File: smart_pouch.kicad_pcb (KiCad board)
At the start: 2 copper layers, 92 parts, among them CN1 B3B-PH-K-S, J1 XH-2P-SMD, J2 2.54-3P-LT, J3 SIM_Card, Q2 PMV20XNER, Q3 2N7002, SW1 SW_Push, U1 nRF52840, U10 BWU.FL-IPEX1, U11 HX PZ1.27-2x5P TP, U12 MT3608, U13 MT3608, U14 HX PZ1.27-2x5P TP, U2 NRF9151-LACA-R7, U3 NPM1300, U4 BMA400, U5 DRV8871DDA, U6 BWU.FL-IPEX1, U7 AN6520-245, U8 SEN0348_CONN, U9 XH-4A, Y1 32MHz

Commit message: Initial PCB commit
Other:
- copper layers 2 -> 4
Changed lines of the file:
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@@
 	(layers
 		(0 "F.Cu" signal)
+		(4 "In1.Cu" signal)
+		(6 "In2.Cu" signal)
 		(2 "B.Cu" signal)
 		(9 "F.Adhes" user "F.Adhesive")
@@
 	)
 	(setup
+		(stackup
+			(layer "F.SilkS"
+				(type "Top Silk Screen")
+			)
+			(layer "F.Paste"
+				(type "Top Solder Paste")
+			)
+			(layer "F.Mask"
+				(type "Top Solder Mask")
+				(thickness 0.01)
+			)
+			(layer "F.Cu"
+				(type "copper")
+				(thickness 0.035)
+			)
+			(layer "dielectric 1"
+				(type "prepreg")
+				(color "FR4 natural")
+				(thickness 0.0994)
+				(material "3313")
+				(epsilon_r 4.1)
+				(loss_tangent 0.02)
+			)
+			(layer "In1.Cu"
+				(type "copper")
+				(thickness 0.0152)
+			)
+			(layer "dielectric 2"
+				(type "core")
+				(color "FR4 natural")
+				(thickness 1.265)
+				(material "FR4")
+				(epsilon_r 4.6)
+				(loss_tangent 0.02)
+			)
+			(layer "In2.Cu"
+				(type "copper")
+				(thickness 0.0152)
+			)
+			(layer "dielectric 3"
+				(type "prepreg")
+				(color "FR4 natural")
+				(thickness 0.0994)
+				(material "3313")
+				(epsilon_r 4.1)
+				(loss_tangent 0.02)
+			)
+			(layer "B.Cu"
+				(type "copper")
+				(thickness 0.035)
+			)
+			(layer "B.Mask"
+				(type "Bottom Solder Mask")
+				(thickness 0.01)
+			)
+			(layer "B.Paste"
+				(type "Bottom Solder Paste")
+			)
+			(layer "B.SilkS"
+				(type "Bottom Silk Screen")
+			)
+			(copper_finish "ENIG")
+			(dielectric_constraints yes)
+		)
 		(pad_to_mask_clearance 0)
 		(allow_soldermask_bridges_in_footprints no)

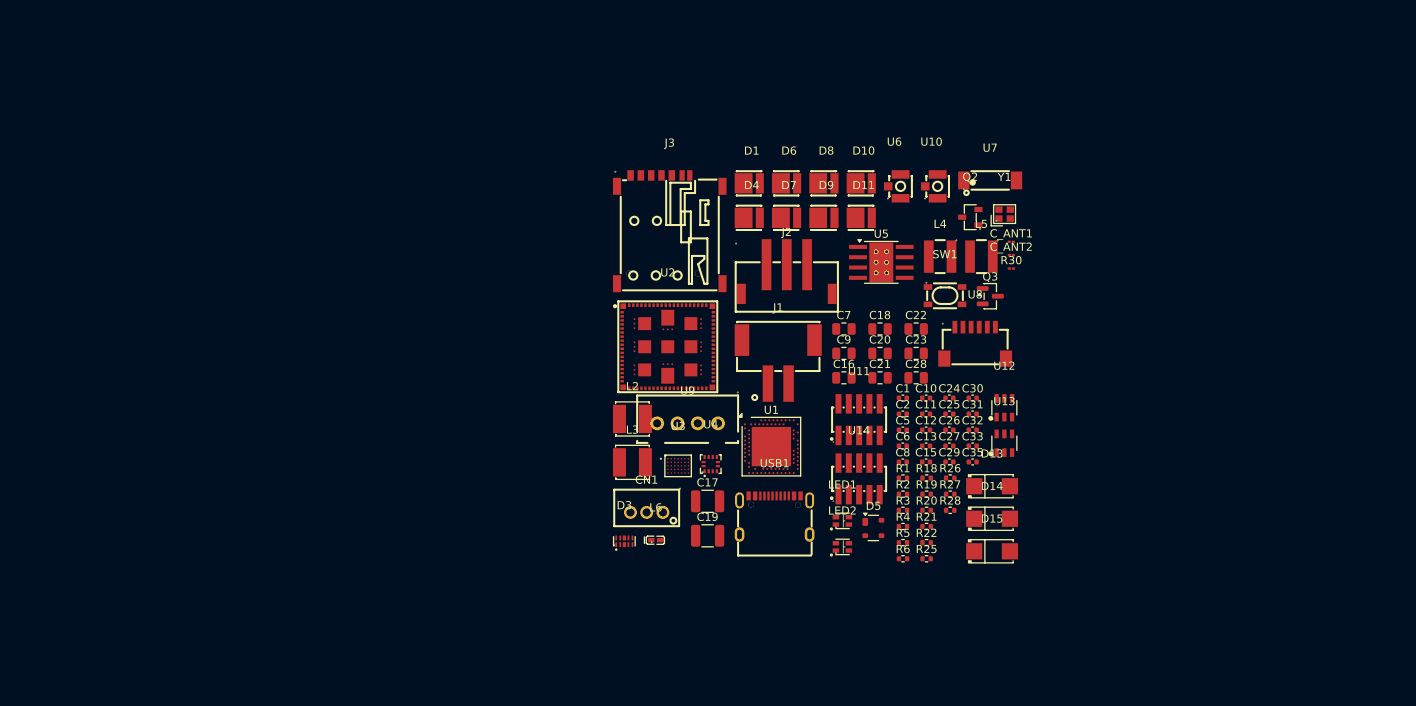
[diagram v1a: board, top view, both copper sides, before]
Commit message: pcb basic layout
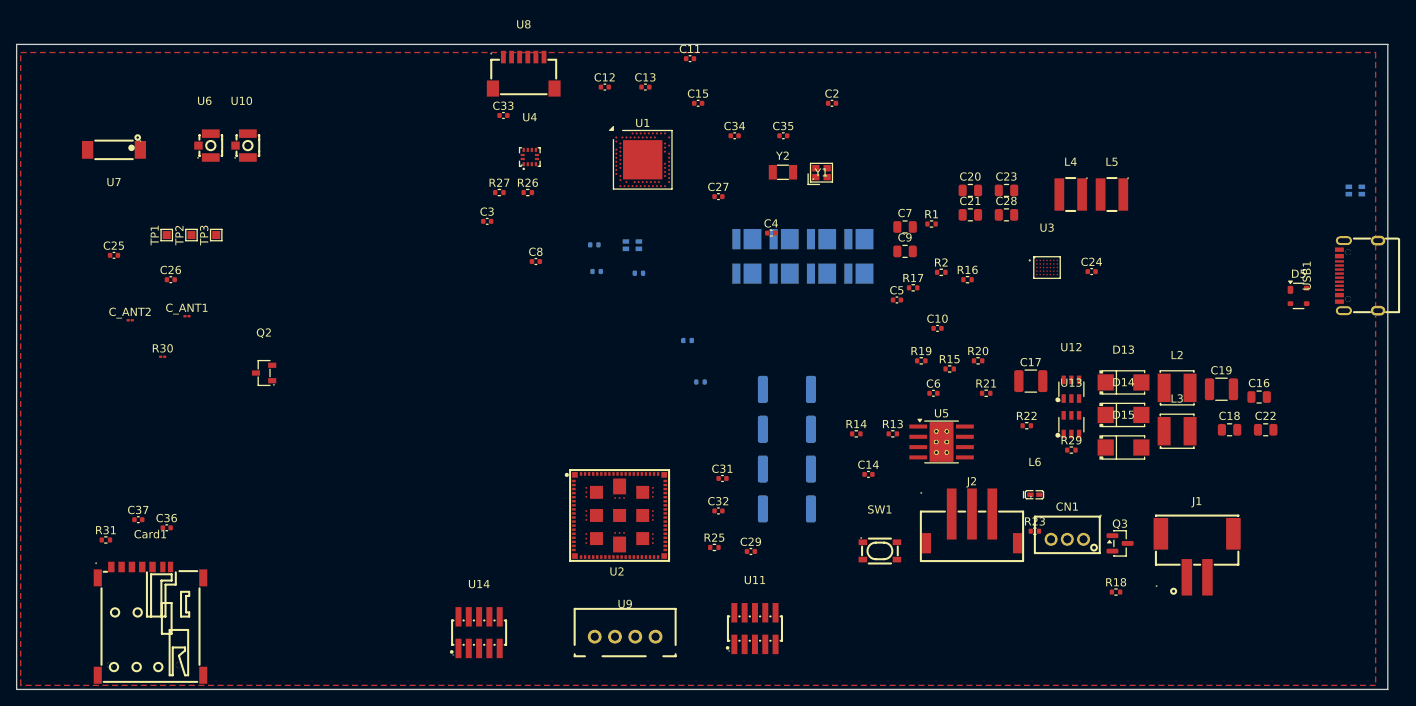
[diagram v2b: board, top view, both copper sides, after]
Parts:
- removed C1, C30: 100nF, Capacitor_SMD:C_0402_1005Metric
- removed D3: SP3012-04UTG, easyeda2kicad:UDFN-10_L2.5-W1.0-P0.50-BL
- removed J3: SIM_Card, easyeda2kicad:SIM-SMD_SMN-303
- removed R3, R4: 10k, Resistor_SMD:R_0402_1005Metric
- added C14: 100nF, Capacitor_SMD:C_0402_1005Metric, F.Cu at (154.0, 102.0)
- added C3: 100nF, Capacitor_SMD:C_0402_1005Metric, F.Cu at (107.0, 70.8)
- added C34: 12pF, Capacitor_SMD:C_0402_1005Metric, F.Cu at (137.5, 60.3)
- added C36: 100nF, Capacitor_SMD:C_0402_1005Metric, F.Cu at (67.5, 108.6)
- added C37: 100nF, Capacitor_SMD:C_0402_1005Metric, F.Cu at (64.0, 107.6)
- added C4: 12pF, Capacitor_SMD:C_0402_1005Metric, F.Cu at (142.0, 72.3)
- added Card1: SMN-303, easyeda2kicad:SIM-SMD_SMN-303, F.Cu at (65.5, 120.1)
- added R10: 39R, Resistor_SMD:R_2512_6332Metric, B.Cu at (143.9, 106.2)
- added R11: 150R, Resistor_SMD:R_0402_1005Metric, B.Cu at (133.3, 90.6)
- added R12: 10k, Resistor_SMD:R_0402_1005Metric, B.Cu at (131.7, 85.5)
- added R13: 560k, Resistor_SMD:R_0402_1005Metric, F.Cu at (157.0, 97.0)
- added R14: 2.2M, Resistor_SMD:R_0402_1005Metric, F.Cu at (152.5, 97.0)
- added R15: 100k, Resistor_SMD:R_0402_1005Metric, F.Cu at (164.0, 89.0)
- added R16: 10k, Resistor_SMD:R_0402_1005Metric, F.Cu at (166.2, 78.0)
- added R17: 10k, Resistor_SMD:R_0402_1005Metric, F.Cu at (159.5, 79.0)
- added R23: 18k, Resistor_SMD:R_0402_1005Metric, F.Cu at (174.5, 109.0)
- added R29: 100k, Resistor_SMD:R_0402_1005Metric, F.Cu at (179.0, 99.0)
- added R31: 10k, Resistor_SMD:R_0402_1005Metric, F.Cu at (60.0, 110.1)
- added R7: 39R, Resistor_SMD:R_2512_6332Metric, B.Cu at (143.9, 91.5)
- added R8: 39R, Resistor_SMD:R_2512_6332Metric, B.Cu at (143.9, 96.4)
- added R9: 39R, Resistor_SMD:R_2512_6332Metric, B.Cu at (143.9, 101.3)
- added TP1: TestPoint, TestPoint:TestPoint_Pad_1.0x1.0mm, F.Cu at (67.5, 72.5)
- added TP2: TestPoint, TestPoint:TestPoint_Pad_1.0x1.0mm, F.Cu at (70.5, 72.5)
- added TP3: TestPoint, TestPoint:TestPoint_Pad_1.0x1.0mm, F.Cu at (73.6, 72.5)
- added Y2: 32.768kHz, Crystal:Crystal_SMD_3215-2Pin_3.2x1.5mm, F.Cu at (143.4, 64.8)
- CN1: value B3B-PH-K-S -> JST 1x3 Battery P=1.27mm
- D1, D10, D11, D4, D6, D7, D8, D9, R28, R5, R6: moved to B.Cu
- D5: value PRTR5V0U2X -> PRTR5V0U2X ESD
- J1: value XH-2P-SMD -> Solenoid XH-2P-SMD
- J2: value 2.54-3P-LT -> 2.54-3P-LT Piezo
- LED1: value 19-237/R6GHBHC-A01/2T -> Power RGB; moved to B.Cu
- LED2: value 19-237/R6GHBHC-A01/2T -> USER LED; moved to B.Cu
- U11: value HX PZ1.27-2x5P TP -> 9151 SWD P=1.27mm 2x5P
- U14: value HX PZ1.27-2x5P TP -> 52840 SWD P=1.27mm 2x5P
- U8: value SEN0348_CONN -> JST P=1mm 01x06
- U9: value XH-4A -> XH-4A UART 9151
- USB1: value TYPE-C 16PIN 2MD -> TYPE-C 16P
- moved C_ANT2 108.9 mm to (63.0, 83.0)
- moved U7 108.1 mm to (61.0, 62.0), turned to 180 degrees
- moved R30 105.2 mm to (67.0, 87.5)
- moved C25 104.8 mm to (61.0, 75.0)
- moved C_ANT1 102.0 mm to (70.0, 82.5)
- moved C26 97.7 mm to (68.0, 78.0)
- moved Q2 89.1 mm to (79.5, 89.5)
- moved U10 85.2 mm to (76.7, 61.5)
- moved U6 85.2 mm to (72.2, 61.5)
- moved USB1 77.8 mm to (214.4, 77.5), turned to 90 degrees
- moved LED1 75.2 mm to (214.0, 67.0), turned to 180 degrees
- moved C33 70.7 mm to (109.0, 57.8)
- moved L2 67.2 mm to (192.0, 91.3)
- moved L3 67.2 mm to (192.0, 96.7)
- moved R27 66.9 mm to (108.5, 67.3)
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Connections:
- U2 pad 26: unconnected-(U2-SIM_DET-Pad26) -> /SIM_CD
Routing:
- added copper zone on F.Cu, net GND
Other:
- board outline added: 169 x 79.5 mm
